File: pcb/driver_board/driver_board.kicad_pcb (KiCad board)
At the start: 2 copper layers, 60 parts, among them J1 Conn_01x02, U1 TJA1051T, U2 AMS1117-3.3

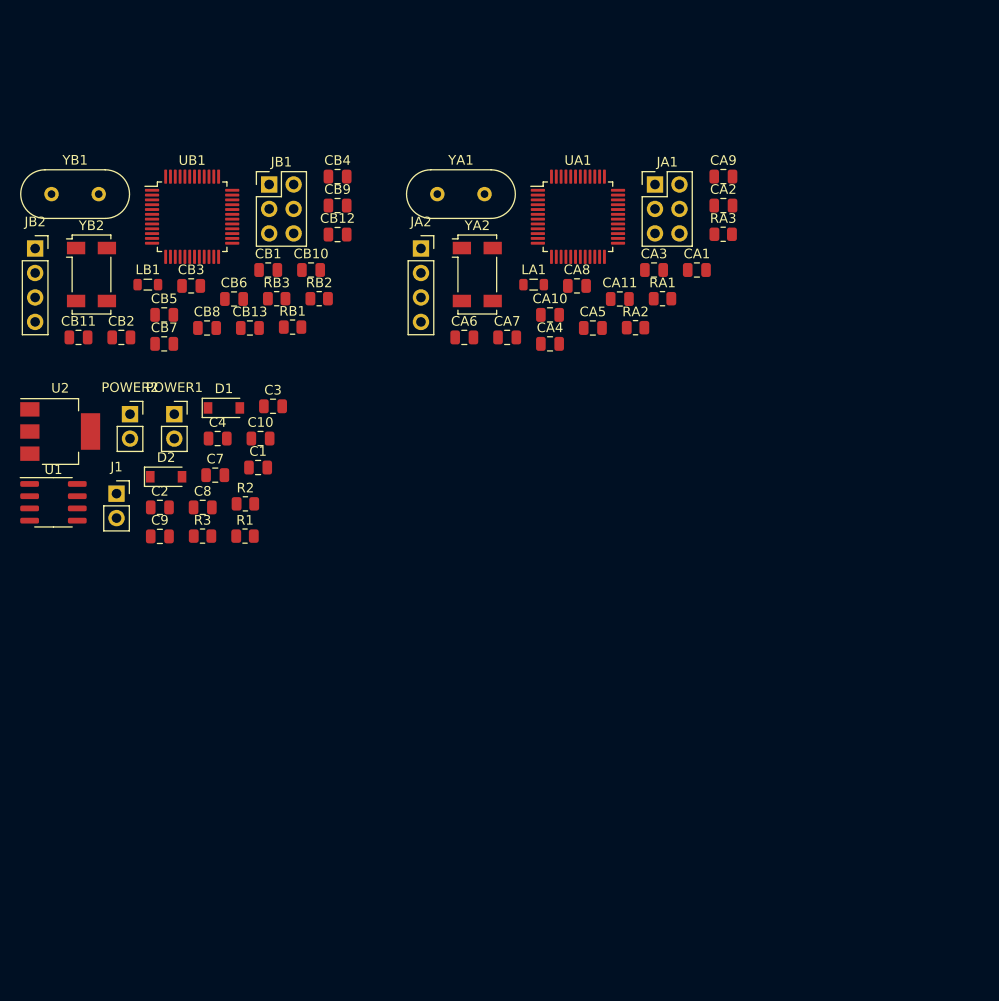
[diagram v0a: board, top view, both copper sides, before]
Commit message: Update layout.
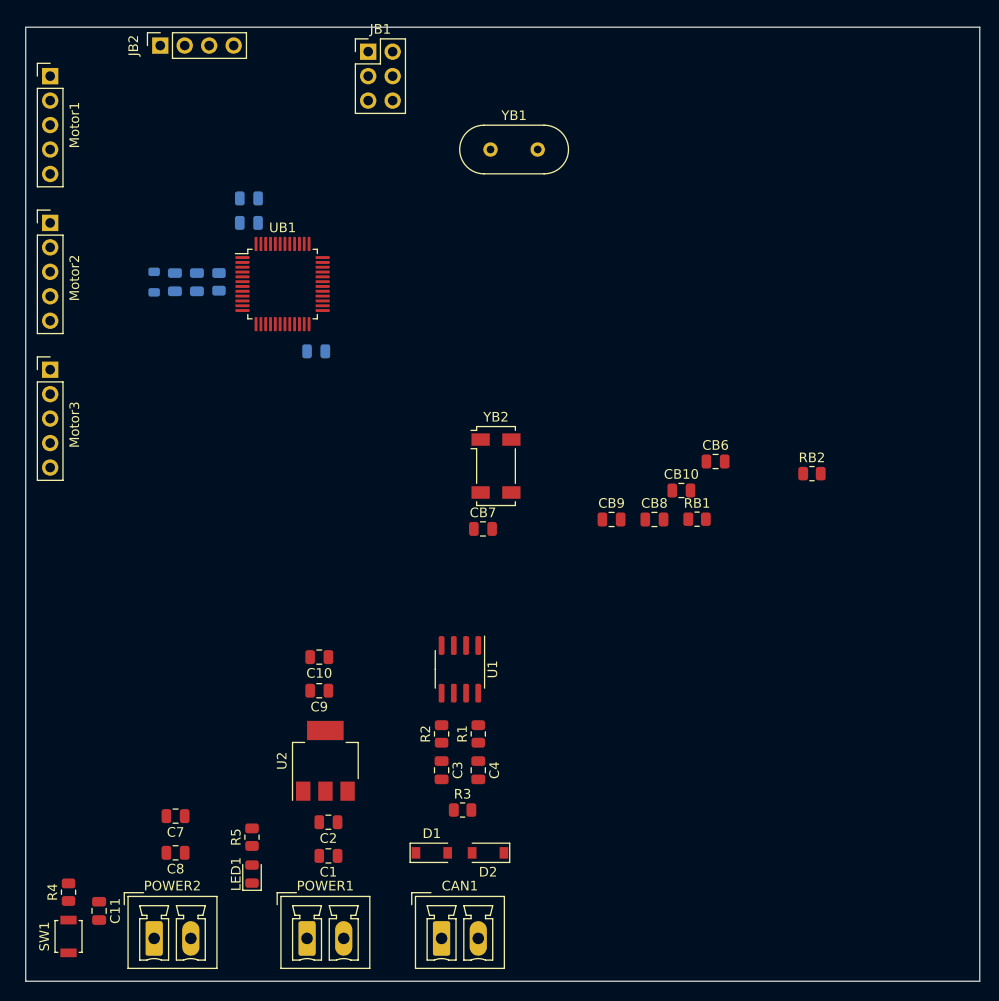
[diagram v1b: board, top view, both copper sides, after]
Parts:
- removed CA1: 4.7uF, Capacitor_SMD:C_0805_2012Metric
- removed CA10, CA11, CA7, CA8, CB11: 20pF, Capacitor_SMD:C_0805_2012Metric
- removed CA2, CB13: 10nF, Capacitor_SMD:C_0805_2012Metric
- removed CA3, CA4, CA5, CA9: 0.1uF, Capacitor_SMD:C_0805_2012Metric
- removed CA6, CB12: 1uF, Capacitor_SMD:C_0805_2012Metric
- removed J1: Conn_01x02, Connector_PinSocket_2.54mm:PinSocket_1x02_P2.54mm_Vertical
- removed JA1: Conn_02x03_Odd_Even, Connector_PinHeader_2.54mm:PinHeader_2x03_P2.54mm_Vertical
- removed JA2: Conn_01x04, Connector_PinSocket_2.54mm:PinSocket_1x04_P2.54mm_Vertical
- removed LA1: 10uH, Inductor_SMD:L_0805_2012Metric
- removed RA1, RA2: 100K, Resistor_SMD:R_0805_2012Metric
- removed RA3: 0R, Resistor_SMD:R_0805_2012Metric
- removed UA1: STM32F103C6Tx, Package_QFP:LQFP-48_7x7mm_P0.5mm
- removed YA1: 8M, Crystal:Crystal_HC18-U_Vertical
- removed YA2: 32768HZ, Crystal:Crystal_SMD_Abracon_ABS25-4Pin_8.0x3.8mm
- added C11: 10pF, Capacitor_SMD:C_0805_2012Metric, F.Cu at (83.8, 129.9)
- added CAN1: Conn_01x02, Connector_Phoenix_MC:PhoenixContact_MCV_1,5_2-G-3.81_1x02_P3.81mm_Vertical, F.Cu at (119.4, 132.7)
- added LED1: LED, LED_SMD:LED_0805_2012Metric, F.Cu at (99.7, 126.0)
- added Motor1: Conn_01x05, Connector_PinHeader_2.54mm:PinHeader_1x05_P2.54mm_Vertical, F.Cu at (78.7, 43.2)
- added Motor2: Conn_01x05, Connector_PinHeader_2.54mm:PinHeader_1x05_P2.54mm_Vertical, F.Cu at (78.7, 58.4)
- added Motor3: Conn_01x05, Connector_PinHeader_2.54mm:PinHeader_1x05_P2.54mm_Vertical, F.Cu at (78.7, 73.7)
- added R4: 10K, Resistor_SMD:R_0805_2012Metric, F.Cu at (80.6, 127.9)
- added R5: 510R, Resistor_SMD:R_0805_2012Metric, F.Cu at (99.7, 122.2)
- added SW1: SW_Push, Button_Switch_SMD:SW_SPST_B3U-1000P, F.Cu at (80.6, 132.5)
- CB1, CB2, CB3, LB1, RB3: moved to B.Cu
- CB4: value 0.1uF -> 1uF; moved to B.Cu
- CB5: value 0.1uF -> 10nF; moved to B.Cu
- CB6, CB9: value 0.1uF -> 20pF
- CB8: value 20pF -> 0.1uF
- POWER1, POWER2: footprint Connector_PinSocket_2.54mm:PinSocket_1x02_P2.54mm_Vertical -> Connector_Phoenix_MC:PhoenixContact_MCV_1,5_2-G-3.81_1x02_P3.81mm_Vertical
- moved POWER1 56.2 mm to (105.4, 132.7)
- moved POWER2 54.5 mm to (89.5, 132.7)
- moved RB2 54.3 mm to (157.8, 84.5)
- moved CB6 52.8 mm to (147.8, 83.2)
- moved D2 51.4 mm to (124.2, 123.8), turned to 180 degrees
- moved D1 51.0 mm to (118.4, 123.8)
- moved CB8 50.5 mm to (141.5, 89.2)
- moved RB1 46.5 mm to (145.9, 89.2)
- moved YB2 46.5 mm to (125.0, 83.7)
- moved YB1 45.8 mm to (124.5, 50.8)
- moved U1 45.6 mm to (121.3, 104.8), turned to 270 degrees
- moved CB10 44.8 mm to (144.3, 86.2)
- moved U2 43.9 mm to (107.3, 114.3), turned to 90 degrees
- moved C4 43.8 mm to (123.2, 115.2), turned to 270 degrees
- moved CB9 43.3 mm to (137.0, 89.2)
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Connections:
- C4 pad 1: /CANL -> /CANH
- C7 pad 2: GND -> GNDA
- C8 pad 2: GND -> GNDA
- CB1 pad 1: /sheet61233186/VDD1 -> +3.3V
- CB10 pad 2: /sheet61233186/RCC_OSC32_IN -> /sheet61233186/RCC_OSC32_OUT
- CB2 pad 1: /sheet61233186/VDD2 -> +3.3V
- CB4 pad 1: +3.3V -> +3.3VA
- CB5 pad 1: +3.3V -> +3.3VA
- CB6 pad 1: /sheet61233186/VDD2 -> Net-(CB6-Pad1)
- CB6 pad 2: GND -> /sheet61233186/RCC_OSC_IN
- CB7 pad 1: Net-(CB7-Pad1) -> Net-(CB6-Pad1)
- CB7 pad 2: /sheet61233186/RCC_OSC_IN -> /sheet61233186/RCC_OSC_OUT
- CB8 pad 1: Net-(CB7-Pad1) -> +3.3V
- CB8 pad 2: /sheet61233186/RCC_OSC_OUT -> Net-(CB8-Pad2)
- CB9 pad 1: +3.3V -> Net-(CB10-Pad1)
- CB9 pad 2: GND -> /sheet61233186/RCC_OSC32_IN
- JB2 pad 1: GND -> Net-(CB8-Pad2)
- POWER2 pad 1: GND -> GNDA
- UB1 pad 11: Net-(UB1-Pad11) -> /sheet61233186/TIM2_CH2
- UB1 pad 13: Net-(UB1-Pad13) -> /sheet61233186/TIM2_CH4
- UB1 pad 15: Net-(UB1-Pad15) -> /sheet61233186/TIM2_CH1
- UB1 pad 18: Net-(UB1-Pad18) -> /sheet61233186/TIM3_CH3
- UB1 pad 19: Net-(UB1-Pad19) -> /sheet61233186/TIM3_CH4
- UB1 pad 21: Net-(UB1-Pad21) -> /sheet61233186/TIM2_CH3
- UB1 pad 24: /sheet61233186/VDD1 -> +3.3V
- UB1 pad 29: Net-(UB1-Pad29) -> /sheet61233186/TIM1_CH1
- UB1 pad 30: Net-(UB1-Pad30) -> /sheet61233186/TIM1_CH2
- UB1 pad 31: Net-(UB1-Pad31) -> /sheet61233186/TIM1_CH3
- UB1 pad 32: Net-(UB1-Pad32) -> /sheet61233186/TIM1_CH4
- UB1 pad 40: Net-(UB1-Pad40) -> /sheet61233186/TIM3_CH1
- UB1 pad 41: Net-(UB1-Pad41) -> /sheet61233186/TIM3_CH2
- UB1 pad 48: /sheet61233186/VDD2 -> +3.3V
- UB1 pad 7: Net-(UB1-Pad7) -> RESET
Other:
- board outline added: 99.1 x 99.1 mm
